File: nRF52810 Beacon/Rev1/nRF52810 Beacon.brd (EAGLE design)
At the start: 27 x 26.8 mm, 19 parts, among them IC1 NRF52810_QF48

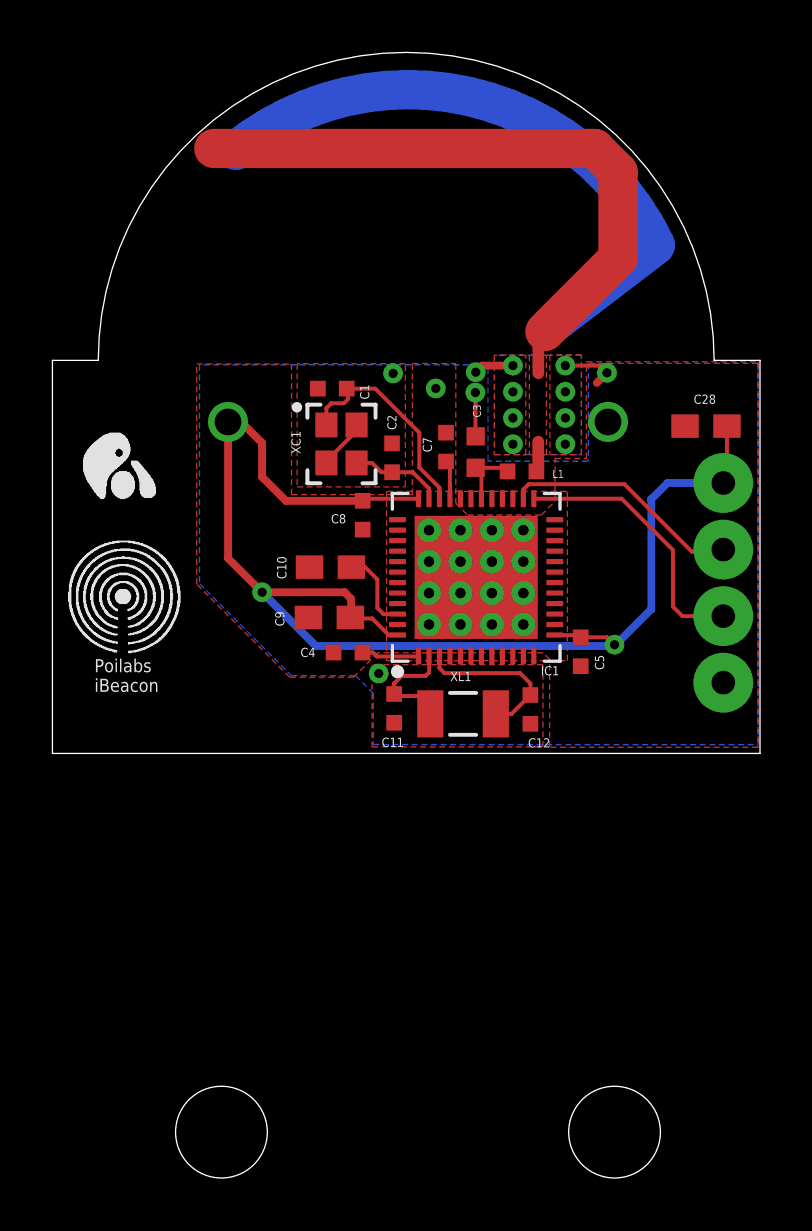
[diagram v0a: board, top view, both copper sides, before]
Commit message: devre revizeleri
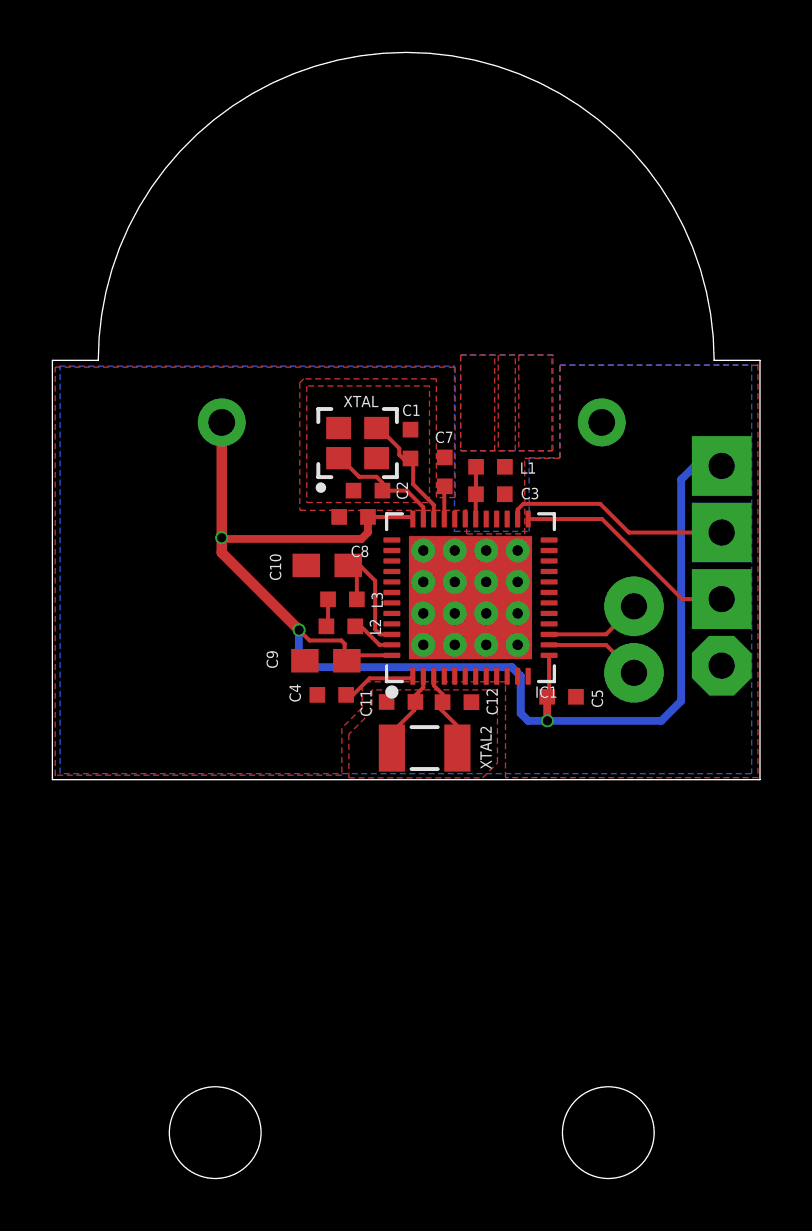
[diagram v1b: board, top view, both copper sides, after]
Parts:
- removed C28: 100nF, Nordic_misc:RESC0603_N
- removed XC1: 32mhz, Nordic_nRF:BT-XTAL_2016_N
- removed XL1: 32.768KHz, Nordic_nRF:XTAL_3215_N
- added L2: 10uH, Nordic_nRF:RESC0402_N
- added L3: 15nH, Nordic_nRF:RESC0402_N
- added XTAL: 32MHz SMD2016, Nordic_nRF:BT-XTAL_2016_N
- added XTAL2: 32KHz, Nordic_nRF:XTAL_3215_N
- C3: device Nordic_nRF:RESC0402_M -> Nordic_nRF:RESC0402_N
- C9: value 1uF -> 4.7uF
- L1: value 3.9nH -> 3.9nF
- U$1: value (none) -> SWD; device 2023Poi:POILOGO -> 2023Poi:SWD
- U$2: value (none) -> UART; device 2023Poi:IBEACON -> 2023Poi:UART
- moved U$1 23.7 mm to (25.5, 11.0), turned to 270 degrees
- moved U$2 19.8 mm to (22.2, 5.62), turned to 270 degrees
- moved C1 3.66 mm to (13.7, 11.8), turned to 270 degrees
- moved C12 2.82 mm to (15.4, 1.96), turned to 180 degrees
- moved C5 1.87 mm to (19.4, 2.16), turned to 0 degrees
- moved C4 1.73 mm to (10.7, 2.23), turned to 0 degrees
- moved C3 1.70 mm to (16.7, 9.89), turned to 0 degrees
- moved C9 1.66 mm to (10.4, 3.54)
- moved C2 1.55 mm to (12.0, 10.0), turned to 0 degrees
- moved L1 1.21 mm to (16.7, 10.9)
- moved C7 0.95 mm to (15.0, 10.7)
- moved IC1 0.81 mm to (16.0, 5.94)
- moved C11 0.36 mm to (13.3, 1.97), turned to 0 degrees
- moved C8 0.36 mm to (11.5, 9.02), turned to 180 degrees
- moved BT1 0.24 mm to (13.7, -14.5)
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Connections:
- net ANT renamed RF
- removed net N$8: C10.2, IC1.46
- new net N$2: L2.2, L3.1
- new net N$4: IC1.47, L2.1
- new net N$6: C4.2, IC1.1
- new net RX: IC1.15, U$2.RX
- new net TX: IC1.14, U$2.TX
- net GND: now also C1.1, C10.2, C2.1, C4.1, U$1.GND, XTAL.2, XTAL.4; no longer C1.2, C10.1, C2.2, C28.2, C4.2, XC1.2, XC1.4
- net N$1: now also C10.1, IC1.46, L3.2; no longer C4.1, IC1.1
- net SWDCLK: now also U$1.SWDCLK
- net SWDIO: now also U$1.SWDIO
- net VDD: now also U$1.VDD; no longer C28.1
- net XC1: now also C1.2, XTAL.3; no longer C1.1, XC1.1
- net XC2: now also C2.2, XTAL.1; no longer C2.1, XC1.3
- net XL1: now also XTAL2.1; no longer XL1.1
- net XL2: now also XTAL2.2; no longer XL1.2
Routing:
- net RF: track 48.0 -> 0.00 mm
- net GND: track 7.37 -> 0.00 mm, vias 15 -> 0
- net RX: track 0.00 -> 3.68 mm
- net TX: track 0.00 -> 3.68 mm
- net XC1: track 8.33 -> 4.68 mm
- net N$8: track 3.14 -> 0.00 mm
- net N$1: track 2.21 -> 5.20 mm
- net XL2: track 6.23 -> 3.38 mm
- net N$6: track 0.00 -> 2.84 mm
- net SWDCLK: track 10.4 -> 8.65 mm, vias 1 -> 0
- net N$4: track 0.00 -> 1.69 mm
- net XL1: track 4.37 -> 2.79 mm
- net XC2: track 3.56 -> 4.64 mm
- net VDD: track 50.9 -> 52.0 mm
- net N$2: track 0.00 -> 1.06 mm
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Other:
- board size 27 x 26.8 mm -> 27 x 27.8 mm
- board text removed: "Poilabs iBeacon"
